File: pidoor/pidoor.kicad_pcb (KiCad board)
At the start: 2 copper layers, 50 x 28 mm, 38 parts, among them P1 PI, P2 PWR, P3 IN0, P4 IN1, P5 IN2, P6 IN3, P7 READER, P8 MAG0, P9 MAG1, Q1 PMN25UN, Q2 PMN25UN, Q3 PMN25UN, Q4 PMN25UN, U1 MAX232, U2 3.3v

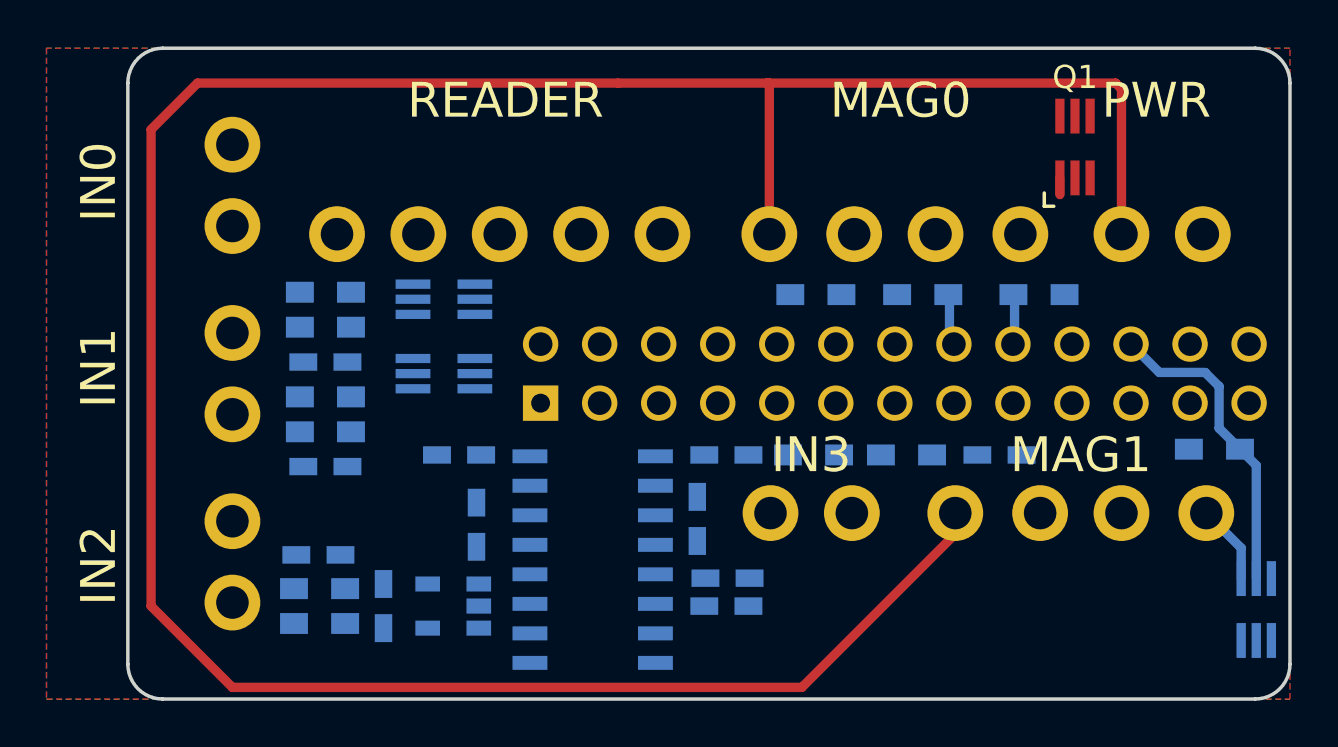
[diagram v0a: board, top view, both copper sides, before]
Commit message: v0.0.1
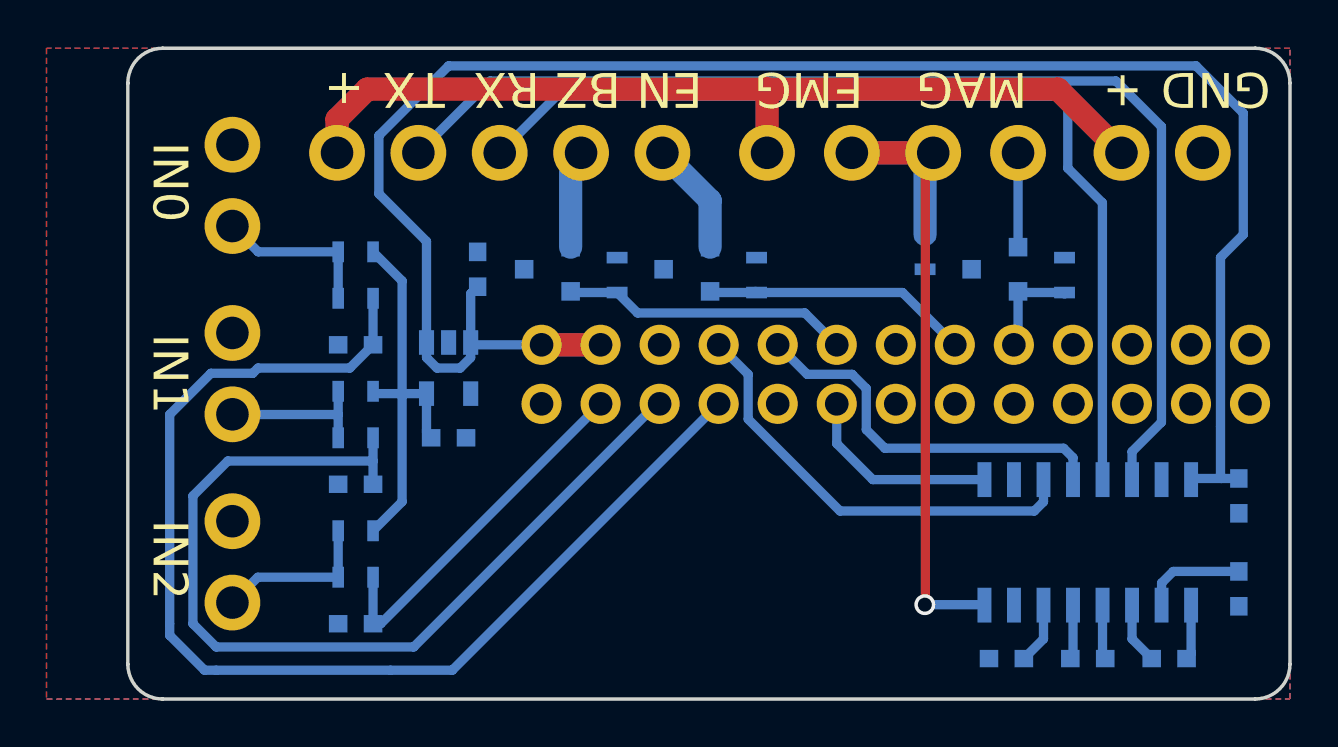
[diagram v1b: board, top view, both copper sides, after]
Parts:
- removed C11: 1µ, Capacitors_SMD:C_0603_HandSoldering
- removed P8: MAG0, pidoor:3_5mm_terminal_1x04
- removed P9: MAG1, pidoor:3_5mm_terminal_1x04
- removed Q4: PMN25UN, TO_SOT_Packages_SMD:SC-70-6_Handsoldering
- removed R11: 1k, Resistors_SMD:R_0603_HandSoldering
- removed R12: 100, Resistors_SMD:R_0603_HandSoldering
- C1, C10, C2, C3, C4, C5, C6, C7, C8, C9: footprint Capacitors_SMD:C_0603_HandSoldering -> Capacitors_SMD:C_0603
- P1: footprint pin_array_13x2 -> Socket_Strips:Socket_Strip_Straight_2x13; moved to B.Cu
- P6: value IN3 -> READER; footprint pidoor:3_5mm_terminal_1x02 -> pidoor:3_5mm_terminal_1x05; moved to B.Cu
- P7: value READER -> MAG; footprint pidoor:3_5mm_terminal_1x05 -> pidoor:3_5mm_terminal_1x04
- Q1: footprint TO_SOT_Packages_SMD:SC-70-6_Handsoldering -> TO_SOT_Packages_SMD:SOT-23; moved to B.Cu
- Q2, Q3: footprint TO_SOT_Packages_SMD:SC-70-6_Handsoldering -> TO_SOT_Packages_SMD:SOT-23
- R1: footprint Resistors_SMD:R_0603_HandSoldering -> Resistors_SMD:R_0603
- R10, R9: value 100 -> 4k7; footprint Resistors_SMD:R_0603_HandSoldering -> Resistors_SMD:R_0603
- R2: value 1k -> 4K7; footprint Resistors_SMD:R_0603_HandSoldering -> Resistors_SMD:R_0603
- R3: value 100 -> 4K7; footprint Resistors_SMD:R_0603_HandSoldering -> Resistors_SMD:R_0603
- R4, R6, R8: value 4K7 -> 4k7; footprint Resistors_SMD:R_0603_HandSoldering -> Resistors_SMD:R_0603
- R5, R7: value 1k -> 4k7; footprint Resistors_SMD:R_0603_HandSoldering -> Resistors_SMD:R_0603
- U1: value MAX232 -> 3.3v; footprint Housings_SOIC:SOIC-16_3.9x9.9mm_Pitch1.27mm -> pidoor:MIC5317
- U2: value 3.3v -> MAX232; footprint TO_SOT_Packages_SMD:SOT-23-5 -> Housings_SOIC:SOIC-16_3.9x9.9mm_Pitch1.27mm
- moved C8 39.6 mm to (175.8, 138.3), turned to 90 degrees
- moved C7 37.2 mm to (172.8, 141.3)
- moved R3 31.1 mm to (137.8, 135.8), turned to 180 degrees
- moved U2 27.4 mm to (169.3, 136.3), turned to 90 degrees
- moved C9 26.9 mm to (169.3, 141.3), turned to 180 degrees
- moved R7 23.1 mm to (155.1, 124.8), turned to 90 degrees
- moved C6 22.6 mm to (175.8, 134.3), turned to 90 degrees
- moved P6 20.5 mm to (144.0, 119.5), turned to 90 degrees
- moved Q3 18.5 mm to (165.3, 124.5), turned to 270 degrees
- moved Q1 17.5 mm to (152.1, 124.5), turned to 270 degrees
- moved P7 17.3 mm to (160.9, 119.5)
- moved C5 15.4 mm to (137.8, 139.8), turned to 180 degrees
- moved P1 15.3 mm to (145.8, 130.3)
- moved R10 15.1 mm to (162.3, 123.8), turned to 270 degrees
- moved C2 13.4 mm to (141.8, 131.8), turned to 0 degrees
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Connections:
- C1 pad 1: Net-(C1-Pad1) -> +5V
- C1 pad 2: Net-(C1-Pad2) -> GND
- C10 pad 1: /GPIO22 -> GND
- C10 pad 2: GND -> Net-(C10-Pad2)
- C2 pad 1: Net-(C2-Pad1) -> +3V3
- C2 pad 2: Net-(C2-Pad2) -> GND
- C3 pad 1: /GPIO4 -> /IN0
- C4 pad 1: GND -> /IN1
- C4 pad 2: +5V -> GND
- C5 pad 1: GND -> /IN2
- C5 pad 2: Net-(C5-Pad2) -> GND
- C6 pad 2: Net-(C6-Pad2) -> +5V
- C7 pad 1: /GPIO17 -> Net-(C7-Pad1)
- C7 pad 2: GND -> Net-(C7-Pad2)
- C8 pad 1: /GPIO21 -> GND
- C8 pad 2: GND -> Net-(C8-Pad2)
- C9 pad 1: +5V -> Net-(C9-Pad1)
- C9 pad 2: GND -> Net-(C9-Pad2)
- P1 pad 1: Net-(P1-Pad1) -> (no net)
- P1 pad 11: /GPIO17 -> /EMG
- P1 pad 12: /GPIO18 -> /BUZZER
- P1 pad 13: /GPIO21 -> (no net)
- P1 pad 14: Net-(P1-Pad14) -> GND
- P1 pad 15: /GPIO22 -> (no net)
- P1 pad 16: /GPIO23 -> /EN_READ
- P1 pad 17: Net-(P1-Pad17) -> (no net)
- P1 pad 18: /GPIO24 -> /MAG
- P1 pad 19: Net-(P1-Pad19) -> (no net)
- P1 pad 20: Net-(P1-Pad20) -> GND
- P1 pad 21: Net-(P1-Pad21) -> (no net)
- P1 pad 22: /GPIO25 -> (no net)
- P1 pad 23: Net-(P1-Pad23) -> (no net)
- P1 pad 24: Net-(P1-Pad24) -> (no net)
- P1 pad 25: Net-(P1-Pad25) -> GND
- P1 pad 26: Net-(P1-Pad26) -> (no net)
- P1 pad 3: Net-(P1-Pad3) -> /IN2
- P1 pad 4: Net-(P1-Pad4) -> +5V
- P1 pad 5: Net-(P1-Pad5) -> /IN1
- P1 pad 7: /GPIO4 -> /IN0
- P1 pad 9: Net-(P1-Pad9) -> GND
- P6 pad 1: GND -> Net-(P6-Pad1)
- P7 pad 2: Net-(P7-Pad2) -> /12_EMG
- P7 pad 3: /EIA-TX -> /12_EMG
- P7 pad 4: /EIA-RX -> +12V
- Q1 pad 1: Net-(P8-Pad1) -> Net-(P6-Pad1)
- Q1 pad 2: /GPIO24 -> /EN_READ
- Q2 pad 1: Net-(P7-Pad1) -> Net-(P6-Pad2)
- Q2 pad 2: /GPIO23 -> /BUZZER
- Q3 pad 1: Net-(P9-Pad1) -> Net-(P7-Pad1)
- Q3 pad 2: /GPIO25 -> /MAG
- R10 pad 1: /GPIO25 -> /12_EMG
- R2 pad 1: /GPIO4 -> +3V3
- R2 pad 2: Net-(P3-Pad2) -> Net-(P4-Pad2)
- R3 pad 1: /GPIO24 -> +3V3
- R3 pad 2: GND -> Net-(P5-Pad2)
- R4 pad 1: +3V3 -> /IN0
- R4 pad 2: Net-(P4-Pad2) -> Net-(P3-Pad2)
- R5 pad 1: /GPIO17 -> /IN1
- R6 pad 1: +3V3 -> /IN2
- R7 pad 1: /GPIO21 -> /EN_READ
- R7 pad 2: Net-(P5-Pad2) -> GND
- R8 pad 1: +3V3 -> /BUZZER
- R8 pad 2: Net-(P6-Pad2) -> GND
- R9 pad 1: /GPIO23 -> /MAG
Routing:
- net +5V: track 0.00 -> 81.7 mm
- net +12V: track 115.7 -> 39.8 mm
- net /IN0: track 0.00 -> 50.5 mm
- net /EIA-TX: track 0.00 -> 49.8 mm
- net /EIA-RX: track 0.00 -> 42.2 mm
- net /IN1: track 0.00 -> 40.7 mm
- net /12_EMG: track 0.00 -> 33.3 mm, vias 0 -> 1
- net /TXD: track 0.00 -> 19.2 mm
- net +3V3: track 0.00 -> 17.4 mm
- net /RXD: track 0.00 -> 16.7 mm
- net /IN2: track 0.00 -> 15.7 mm
- net /GPIO25: track 13.5 -> 0.00 mm
- net /BUZZER: track 0.00 -> 12.4 mm
- net /EN_READ: track 0.00 -> 11.8 mm
- net /EMG: track 0.00 -> 8.71 mm
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- added copper zone on F.Cu, net GND
- removed copper zone on F.Cu, net +3V3
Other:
- net class Default: via_dia 0.9 -> 1
- net class Power: trace_width 0.5 -> 1
- board text added: "+"
- board text added: "BZ"
- board text added: "EMG"
- board text added: "EN"
- board text added: "GND"
- board text added: "IN0"
- board text added: "IN1"
- board text added: "IN2"
- board text added: "MAG"
- board text added: "RX"
- board text added: "TX"
